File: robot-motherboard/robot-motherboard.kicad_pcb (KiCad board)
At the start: 2 copper layers, 30.5 x 53.3 mm, 1 part, among them U1 ESP32_PICO-1

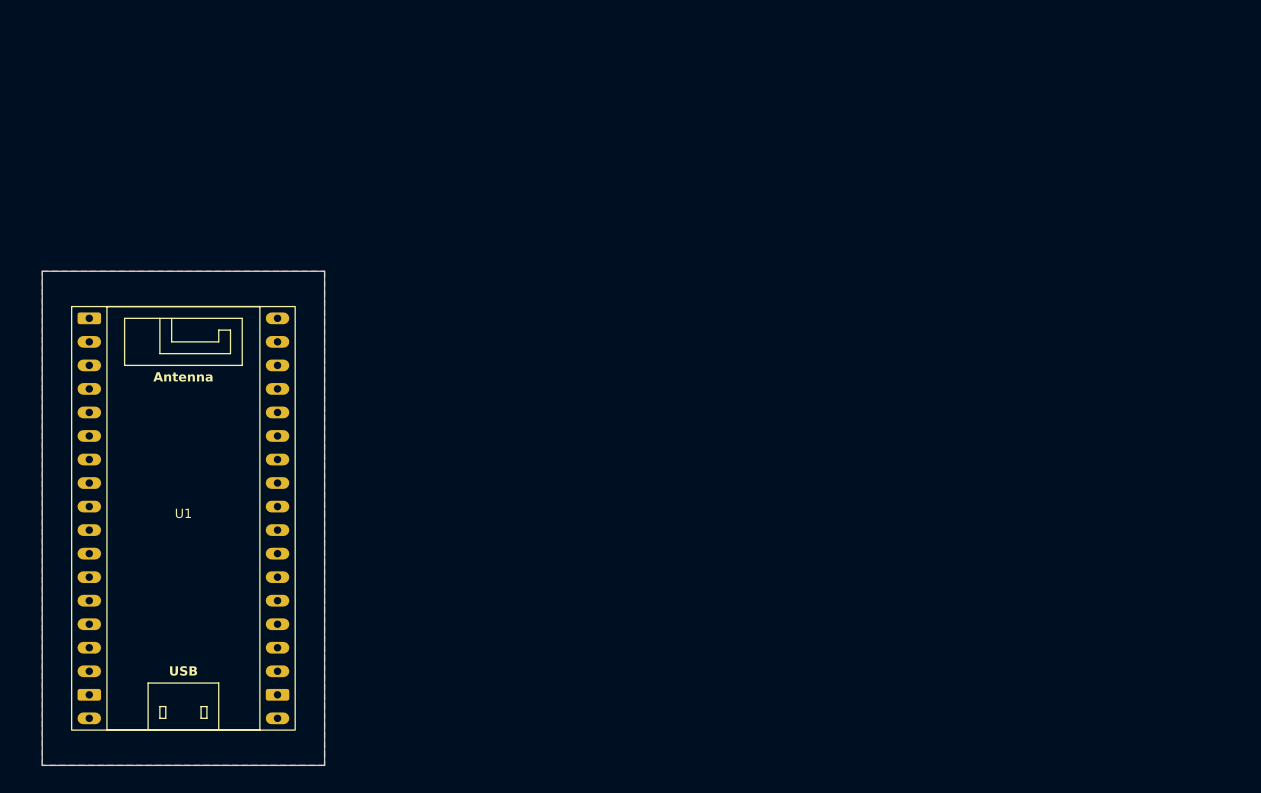
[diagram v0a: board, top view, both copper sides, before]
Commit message: Finish layout
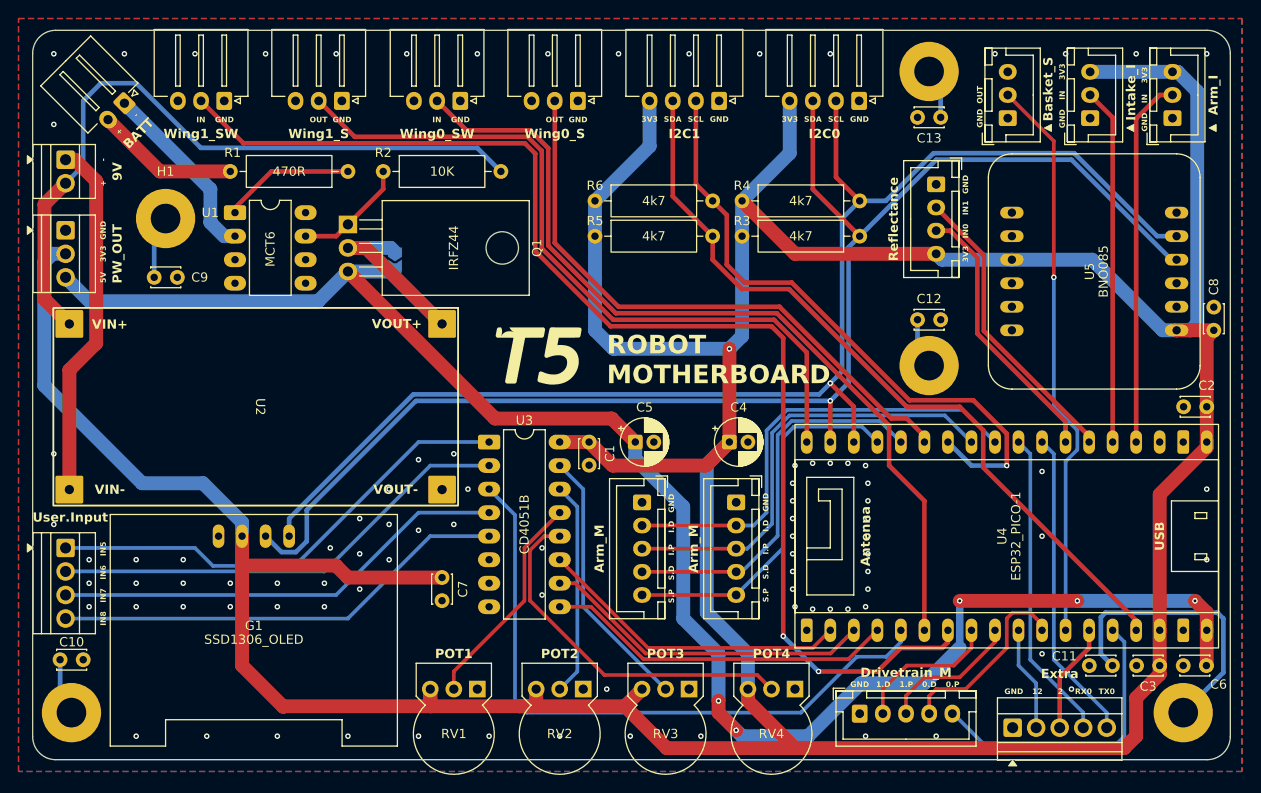
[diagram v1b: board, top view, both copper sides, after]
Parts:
- added C1: 100nF, Capacitor_THT:C_Disc_D3.0mm_W2.0mm_P2.50mm, F.Cu at (191.1, 79.4)
- added C10: 100nF, Capacitor_THT:C_Disc_D3.0mm_W2.0mm_P2.50mm, F.Cu at (134.0, 102.9)
- added C11: 100nF, Capacitor_THT:C_Disc_D3.0mm_W2.0mm_P2.50mm, F.Cu at (247.6, 103.5)
- added C12: 100nF, Capacitor_THT:C_Disc_D3.0mm_W2.0mm_P2.50mm, F.Cu at (226.6, 66.2)
- added C13: 100nF, Capacitor_THT:C_Disc_D3.0mm_W2.0mm_P2.50mm, F.Cu at (229.1, 44.3)
- added C2: 100nF, Capacitor_THT:C_Disc_D3.0mm_W2.0mm_P2.50mm, F.Cu at (257.8, 75.6)
- added C3: 100nF, Capacitor_THT:C_Disc_D3.0mm_W2.0mm_P2.50mm, F.Cu at (252.7, 103.5)
- added C4: 47uF, Capacitor_THT:CP_Radial_D5.0mm_P2.00mm, F.Cu at (206.3, 79.4)
- added C5: 47uF, Capacitor_THT:CP_Radial_D5.0mm_P2.00mm, F.Cu at (196.1, 79.4)
- added C6: 100nF, Capacitor_THT:C_Disc_D3.0mm_W2.0mm_P2.50mm, F.Cu at (257.8, 103.5)
- added C7: 100nF, Capacitor_THT:C_Disc_D3.0mm_W2.0mm_P2.50mm, F.Cu at (175.2, 94.0)
- added C8: 100nF, Capacitor_THT:C_Disc_D3.0mm_W2.0mm_P2.50mm, F.Cu at (258.6, 67.3)
- added C9: 100nF, Capacitor_THT:C_Disc_D3.0mm_W2.0mm_P2.50mm, F.Cu at (144.2, 61.6)
- added G1: SSD1306_OLED, GS_Development_Boards:ADAFRUIT_SSD1306_OLED, F.Cu at (154.9, 99.7)
- added H1: M3_PTH, MountingHole:MountingHole_3.2mm_M3_Pad, F.Cu at (145.4, 55.3)
- added H2: M3_PTH, MountingHole:MountingHole_3.2mm_M3_Pad, F.Cu at (135.2, 108.6)
- added H3: M3_PTH, MountingHole:MountingHole_3.2mm_M3_Pad, F.Cu at (255.2, 108.6)
- added H4: M3_PTH, MountingHole:MountingHole_3.2mm_M3_Pad, F.Cu at (227.8, 71.1)
- added H5: M3_PTH, MountingHole:MountingHole_3.2mm_M3_Pad, F.Cu at (227.8, 39.4)
- added J1: Wing0_S, GS_Connectors:JST_XH_S3B-XH-A-1_1x03_P2.50mm_Horizontal, F.Cu at (189.9, 42.6)
- added J10: Reflectance, Connector_JST:JST_XH_B4B-XH-A_1x04_P2.50mm_Vertical, F.Cu at (228.6, 51.6)
- added J11: Arm_I, Connector_JST:JST_XH_B3B-XH-A_1x03_P2.50mm_Vertical, F.Cu at (254.1, 44.4)
- added J12: Intake_I, Connector_JST:JST_XH_B3B-XH-A_1x03_P2.50mm_Vertical, F.Cu at (245.2, 44.4)
- added J13: User.Input, TerminalBlock:TerminalBlock_Xinya_XY308-2.54-4P_1x04_P2.54mm_Horizontal, F.Cu at (134.6, 90.8)
- added J14: I2C0, GS_Connectors:JST_XH_S4B-XH-A-1_1x04_P2.50mm_Horizontal, F.Cu at (220.3, 42.6)
- added J15: Extra, TerminalBlock:TerminalBlock_Xinya_XY308-2.54-5P_1x05_P2.54mm_Horizontal, F.Cu at (236.8, 110.2)
- added J16: I2C1, GS_Connectors:JST_XH_S4B-XH-A-1_1x04_P2.50mm_Horizontal, F.Cu at (205.1, 42.6)
- added J17: PW_OUT, TerminalBlock:TerminalBlock_Xinya_XY308-2.54-3P_1x03_P2.54mm_Horizontal, F.Cu at (134.6, 56.5)
- added J19: Basket_S, Connector_JST:JST_XH_B3B-XH-A_1x03_P2.50mm_Vertical, F.Cu at (236.3, 44.4)
- added J2: Wing0_SW, GS_Connectors:JST_XH_S3B-XH-A-1_1x03_P2.50mm_Horizontal, F.Cu at (177.2, 42.6)
- added J3: BATT, GS_Connectors:JST_XH_S2B-XH-A-1_1x02_P2.50mm_Horizontal, F.Cu at (140.9, 42.8)
- added J4: Wing1_S, GS_Connectors:JST_XH_S3B-XH-A-1_1x03_P2.50mm_Horizontal, F.Cu at (164.4, 42.6)
- added J5: Wing1_SW, GS_Connectors:JST_XH_S3B-XH-A-1_1x03_P2.50mm_Horizontal, F.Cu at (151.7, 42.6)
- added J6: 9V, TerminalBlock:TerminalBlock_Xinya_XY308-2.54-2P_1x02_P2.54mm_Horizontal, F.Cu at (134.6, 48.9)
- added J7: Drivetrain_M, Connector_JST:JST_XH_B5B-XH-A_1x05_P2.50mm_Vertical, F.Cu at (220.3, 108.7)
- added J8: Arm_M, Connector_JST:JST_XH_B5B-XH-A_1x05_P2.50mm_Vertical, F.Cu at (207.0, 85.9)
- added J9: Arm_M, Connector_JST:JST_XH_B5B-XH-A_1x05_P2.50mm_Vertical, F.Cu at (196.8, 85.9)
- added JP1: Battery bypass, Jumper:SolderJumper-2_P1.3mm_Open_TrianglePad1.0x1.5mm, B.Cu at (170.2, 59.6)
- added Q1: IRFZ44, Package_TO_SOT_THT:TO-220-3_Horizontal_TabDown, F.Cu at (165.1, 55.9)
- added R1: 470R, Resistor_THT:R_Axial_DIN0309_L9.0mm_D3.2mm_P12.70mm_Horizontal, F.Cu at (165.1, 50.2)
- added R2: 10K, Resistor_THT:R_Axial_DIN0309_L9.0mm_D3.2mm_P12.70mm_Horizontal, F.Cu at (168.9, 50.2)
- added R3: 4k7, Resistor_THT:R_Axial_DIN0309_L9.0mm_D3.2mm_P12.70mm_Horizontal, F.Cu at (207.6, 57.2)
- added R4: 4k7, Resistor_THT:R_Axial_DIN0309_L9.0mm_D3.2mm_P12.70mm_Horizontal, F.Cu at (207.6, 53.4)
- added R5: 4k7, Resistor_THT:R_Axial_DIN0309_L9.0mm_D3.2mm_P12.70mm_Horizontal, F.Cu at (191.8, 57.2)
- added R6: 4k7, Resistor_THT:R_Axial_DIN0309_L9.0mm_D3.2mm_P12.70mm_Horizontal, F.Cu at (191.8, 53.4)
- added RV1: POT1, GS_Resistors:ENPH253_Potentiometer, F.Cu at (176.5, 106.1)
- added RV2: POT2, GS_Resistors:ENPH253_Potentiometer, F.Cu at (187.9, 106.1)
- added RV3: POT3, GS_Resistors:ENPH253_Potentiometer, F.Cu at (199.4, 106.1)
- added RV4: POT4, GS_Resistors:ENPH253_Potentiometer, F.Cu at (210.8, 106.1)
- added S1: Logo, GS_Virtual:ENPH253_Logo, F.Cu at (186.0, 69.9)
- added U1: MCT6, Package_DIP:DIP-8_W7.62mm_LongPads, F.Cu at (152.9, 54.6)
- added U2: LM2596_Breakout, GS_Development_Boards:LM2596_Breakout, F.Cu at (155.1, 75.6)
- added U3: CD4051B, Package_DIP:DIP-16_W7.62mm_LongPads, F.Cu at (180.3, 79.4)
- added U5: BNO085, GS_Development_Boards:ADAFRUIT_BNO085, F.Cu at (245.6, 61.0)
- moved U4 88.9 mm to (236.2, 89.6), turned to 90 degrees
- renumbered U1 to U4
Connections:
- U4 pad 1: unconnected-(U1-TX0-Pad1) -> /TX0
- U4 pad 10: unconnected-(U1-GPIO10-Pad10) -> /ARM.INTAKE_PWM
- U4 pad 12: unconnected-(U1-GPIO12-Pad12) -> /GPIO12
- U4 pad 13: unconnected-(U1-GPIO13-Pad13) -> /DRIVETRAIN.M0_DIR
- U4 pad 14: unconnected-(U1-GPIO14-Pad14) -> /DRIVETRAIN.M1_PWM
- U4 pad 15: unconnected-(U1-GPIO15-Pad15) -> /BASKET.SERVO
- U4 pad 19: /M0.DIR -> /ARM.SHOULDER_PWM
- U4 pad 2: unconnected-(U1-GPIO2-Pad2) -> /GPIO2
- U4 pad 20: /M0.PWM -> /WING1.SERVO
- U4 pad 25: unconnected-(U1-GPIO25-Pad25) -> /INPUT.SELECT2
- U4 pad 26: unconnected-(U1-GPIO26-Pad26) -> /INPUT.MCU_IN
- U4 pad 27: unconnected-(U1-GPIO27-Pad27) -> /DRIVETRAIN.M1_DIR
- U4 pad 3: unconnected-(U1-RX0-Pad3) -> /RX0
- U4 pad 32: unconnected-(U1-GPIO32-Pad32) -> /WING0.LIMIT_SW_IN
- U4 pad 33: unconnected-(U1-GPIO33-Pad33) -> /WING1.LIMIT_SW_IN
- U4 pad 34: /M2.DIR -> /IR1.IN
- U4 pad 35: /M2.PWM -> /IR0.IN
- U4 pad 37: /M3.DIR -> /ARM.POSITION
- U4 pad 38: /M3.PWM -> /ARM.INTAKE_SW
- U4 pad 3V3: unconnected-(U1-Pad3V3) -> +3V3
- U4 pad 4: unconnected-(U1-GPIO4-Pad4) -> /DRIVETRAIN.M0_PWM
- U4 pad 5V: unconnected-(U1-Pad5V) -> +5V
- U4 pad 7: /M1.DIR -> /WING0.SERVO
- U4 pad 8: /M1.PWM -> /ARM.SHOULDER_DIR
- U4 pad 9: unconnected-(U1-GPIO9-Pad9) -> /ARM.INTAKE_DIR
- U4 pad VN: unconnected-(U1-GPIO39-PadVN) -> /INPUT.SELECT1
- U4 pad VP: unconnected-(U1-GPIO36-PadVP) -> /INPUT.SELECT0
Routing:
- net +3V3: track 0.00 -> 475.7 mm, vias 0 -> 1
- net +5V: track 0.00 -> 178.6 mm, vias 0 -> 5
- net /I2C0.SDA: track 0.00 -> 152.7 mm, vias 0 -> 1
- net /I2C0.SCL: track 0.00 -> 146.7 mm, vias 0 -> 1
- net /WING1.LIMIT_SW_IN: track 0.00 -> 133.7 mm, vias 0 -> 2
- net /WING0.LIMIT_SW_IN: track 0.00 -> 93.2 mm
- net /I2C1.SDA: track 0.00 -> 84.2 mm
- net /WING1.SERVO: track 0.00 -> 79.8 mm
- net +9V: track 0.00 -> 76.7 mm
- net /INPUT.MCU_IN: track 0.00 -> 70.6 mm
- net /I2C1.SCL: track 0.00 -> 67.7 mm, vias 0 -> 1
- net /WING0.SERVO: track 0.00 -> 64.5 mm
- net /BASKET.SERVO: track 0.00 -> 61.4 mm, vias 0 -> 1
- net Net-(J13-Pin_1): track 0.00 -> 52.1 mm
- net Net-(J13-Pin_2): track 0.00 -> 50.5 mm
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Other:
- board size 30.5 x 53.3 mm -> 129.3 x 78.7 mm
- board text added: "+"
- board text added: "-"
- board text added: "0"
- board text added: "0 mm"
- board text added: "0.01 mm"
- board text added: "0.02"
- board text added: "0.035 mm"
- board text added: "0.1000 mm / 0.1000 mm"
- board text added: "0.3000 mm"
- board text added: "0.D"
- board text added: "0.P"
- board text added: "1"
- board text added: "1.51 mm"
- board text added: "1.6000 mm"
- board text added: "1.D"
- board text added: "1.P"
- board text added: "12"
- board text added: "129.2860 mm x 78.7400 mm"
- board text added: "2"
- board text added: "3.3"
- board text added: "3V3"
- board text added: "4.5"
- board text added: "5V"
- board text added: "B.Cu"
- board text added: "B.Mask"
- board text added: "B.Paste"
- board text added: "B.Silkscreen"
- board text added: "BATT"
- board text added: "BOARD CHARACTERISTICS"
- board text added: "Board Thickness:"
- board text added: "Board overall dimensions:"
- board text added: "Bottom Silk Screen"
- board text added: "Bottom Solder Mask"
- board text added: "Bottom Solder Paste"
- board text added: "Castellated pads:"
- board text added: "Color"
- board text added: "Copper Finish:"
- board text added: "Copper Layer Count:"
- board text added: "Designed by George Sleen"
- board text added: "Dielectric"
- board text added: "Edge card connectors:"
- board text added: "Epsilon R"
- board text added: "F.Cu"
- board text added: "F.Mask"
- board text added: "F.Paste"
- board text added: "F.Silkscreen"
- board text added: "FR4"
- board text added: "GND"
- board text added: "I.D"
- board text added: "I.P"
- board text added: "IN"
- board text added: "IN0"
- board text added: "IN1"
- board text added: "IN5"
- board text added: "IN6"
- board text added: "IN7"
- board text added: "IN8"
- board text added: "Impedance Control:"
- board text added: "Layer Name"
- board text added: "Loss Tangent"
- board text added: "Material"
- board text added: "Min hole diameter:"
- board text added: "Min track/spacing:"
- board text added: "No"
- board text added: "None"
- board text added: "Not specified"
- board text added: "OUT"
- board text added: "PIN STRAPPING: GPIO0 -> PULL-UP GPIO2 -> PULL-DOWN MDTI(GPIO12) -> PULL-DOWN MDTO(GPIO15) -> PULL-UP GPIO5 -> PULL-UP"
- board text added: "Plated Board Edge:"
- board text added: "ROBOT MOTHERBOARD"
- board text added: "RX0"
- board text added: "S.D"
- board text added: "S.P"
- board text added: "SCL"
- board text added: "SDA"
- board text added: "TX0"
- board text added: "Thickness (mm)"
- board text added: "Top Silk Screen"
- board text added: "Top Solder Mask"
- board text added: "Top Solder Paste"
- board text added: "Type"
- board text added: "copper"
- board text added: "core"
- board text added: "github.com /enph253-2025-team5/ robot-motherboard-pcb"
